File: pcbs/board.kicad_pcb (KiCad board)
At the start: 2 copper layers, 120.3 x 95.9 mm, 68 parts

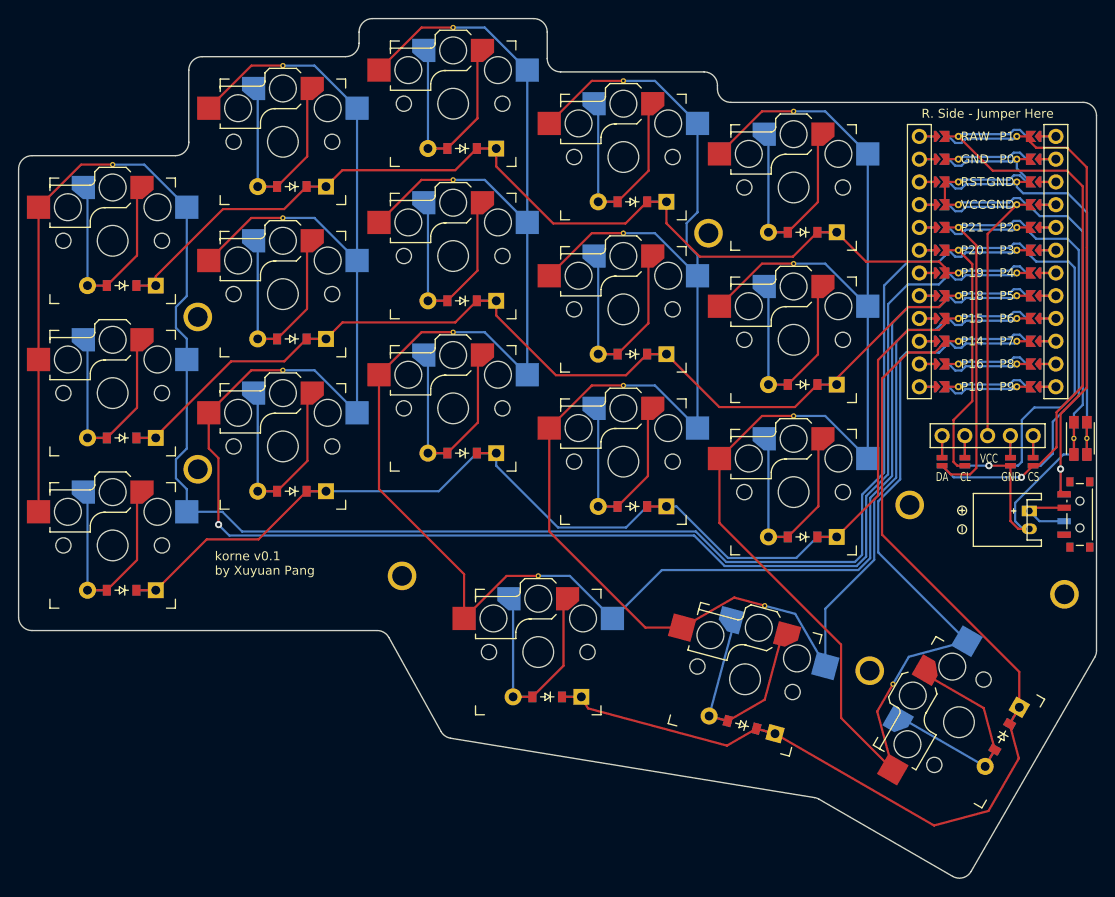
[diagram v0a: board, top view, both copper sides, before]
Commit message: chore: release v0.2
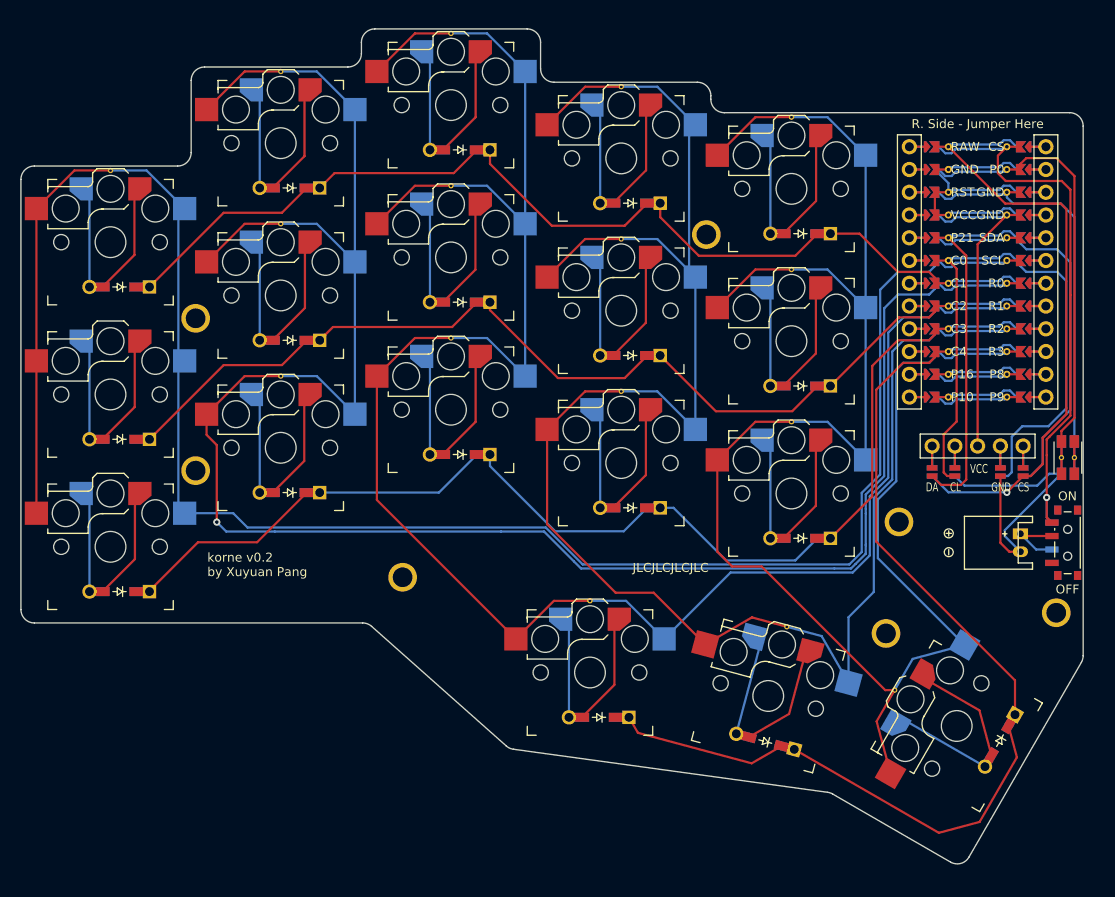
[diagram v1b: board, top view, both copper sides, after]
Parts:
- removed the REF** at (72.6, 8.63)
- removed the REF** at (37.9, -55.9)
- removed the REF** at (75.9, -12.5)
- removed the REF** at (56.9, -49.9)
- removed the REF** at (56.9, -32.9)
- removed the REF** at (18.9, -17.6)
- removed the REF** at (47.4, 5.30)
- removed the REF** at (37.9, -38.9)
- removed the REF** at (37.9, -21.9)
- removed the REF** at (18.9, -34.6)
- removed the REF** at (75.9, -29.5)
- removed the REF** at (56.9, -15.9)
- removed the REF** at (18.9, -51.6)
- removed the REF** at (75.9, -46.5)
- removed the REF** at (108.6, -10.0)
- removed the REF** at (107.1, -10.0)
- removed the REF** at (-0.15, -40.6)
- removed the REF** at (86.9, 17.4)
- added REF**: VIA-0.6mm, VIA-0.6mm, F.Cu at (18.6, -17.0)
- added REF**: VIA-0.6mm, VIA-0.6mm, F.Cu at (18.6, -34.0)
- added REF**: VIA-0.6mm, VIA-0.6mm, F.Cu at (37.6, -38.2)
- added REF**: VIA-0.6mm, VIA-0.6mm, F.Cu at (75.6, -45.9)
- added REF**: VIA-0.6mm, VIA-0.6mm, F.Cu at (56.6, -49.3)
- added REF**: VIA-0.6mm, VIA-0.6mm, F.Cu at (75.1, 11.0)
- added REF**: VIA-0.6mm, VIA-0.6mm, F.Cu at (56.6, -15.3)
- added REF**: VIA-0.6mm, VIA-0.6mm, F.Cu at (107.2, -7.90)
- added REF**: VIA-0.6mm, VIA-0.6mm, F.Cu at (-0.39, -39.9)
- added REF**: VIA-0.6mm, VIA-0.6mm, F.Cu at (53.1, 8.09)
- added REF**: VIA-0.6mm, VIA-0.6mm, F.Cu at (56.6, -32.3)
- added REF**: VIA-0.6mm, VIA-0.6mm, F.Cu at (75.6, -11.9)
- added REF**: VIA-0.6mm, VIA-0.6mm, F.Cu at (18.6, -51.0)
- added REF**: VIA-0.6mm, VIA-0.6mm, F.Cu at (37.6, -21.2)
- added REF**: VIA-0.6mm, VIA-0.6mm, F.Cu at (75.6, -28.9)
- added REF**: VIA-0.6mm, VIA-0.6mm, F.Cu at (37.6, -55.2)
- added REF**: VIA-0.6mm, VIA-0.6mm, F.Cu at (87.1, 18.1)
- added REF**: VIA-0.6mm, VIA-0.6mm, F.Cu at (105.7, -7.90)
- moved D16 50.8 mm to (98.9, 23.7), turned to -120 degrees
- moved D18 45.1 mm to (54.1, 21.1), turned to 180 degrees
- moved S16 26.1 mm to (73.0, 18.7), turned to -15 degrees
- moved S17 17.3 mm to (53.1, 16.1), turned to 0 degrees
- moved H5 4.54 mm to (86.2, 11.7)
- moved SW2 3.44 mm to (106.4, 1.60)
- moved D17 3.19 mm to (72.7, 23.8)
- moved ? 2.96 mm to (93.2, 1.60)
- moved ICON1 2.96 mm to (93.2, 1.60)
- moved JST1 2.74 mm to (101.2, 1.60)
- moved SW1 2.56 mm to (106.5, -7.90)
- moved H6 2.25 mm to (105.2, 9.42), turned to 30 degrees
- moved H7 2.24 mm to (87.6, -0.72), turned to -60 degrees
- moved MCU1 1.60 mm to (96.4, -29.9)
- moved DISP1 1.60 mm to (96.4, -25.9)
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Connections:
- D16 pad 2: near_thumb -> far_thumb
- D18 pad 2: far_thumb -> near_thumb
- S16 pad 1: near_thumb -> home_thumb
- S16 pad 2: col_middle -> col_index
- S17 pad 1: home_thumb -> near_thumb
- S17 pad 2: col_index -> col_middle
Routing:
- net row_top: track 131.1 -> 110.8 mm
- net row_home: track 131.3 -> 111.2 mm
- net row_bottom: track 145.4 -> 125.8 mm
- net row_thumb: track 133.8 -> 115.8 mm
- net GND: track 98.8 -> 116.4 mm, vias 1 -> 0
- net col_inner: track 211.6 -> 202.0 mm
- net RAW: track 59.1 -> 63.9 mm
- net col_middle: track 223.6 -> 219.5 mm
- net inner_home: track 28.0 -> 24.0 mm
- net ring_top: track 28.0 -> 24.0 mm
- net far_thumb: track 28.0 -> 24.0 mm
- net index_bottom: track 28.0 -> 24.0 mm
- net index_home: track 28.0 -> 24.0 mm
- net home_thumb: track 28.0 -> 24.0 mm
- net middle_home: track 28.0 -> 24.0 mm
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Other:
- board size 120.3 x 95.9 mm -> 118.6 x 93.2 mm
- board text added: "JLCJLCJLCJLC"
- board text added: "OFF"
- board text added: "ON"
- board text added: "korne v0.2 by Xuyuan Pang"
- board text removed: "korne v0.1 by Xuyuan Pang"
